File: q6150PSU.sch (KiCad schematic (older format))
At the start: 25 parts, among them P1 Vin, P2 Vout, P3 CONN_01X03, Q1 Q_NMOS_GSD, T1 TRANSFO, U1 LM3478

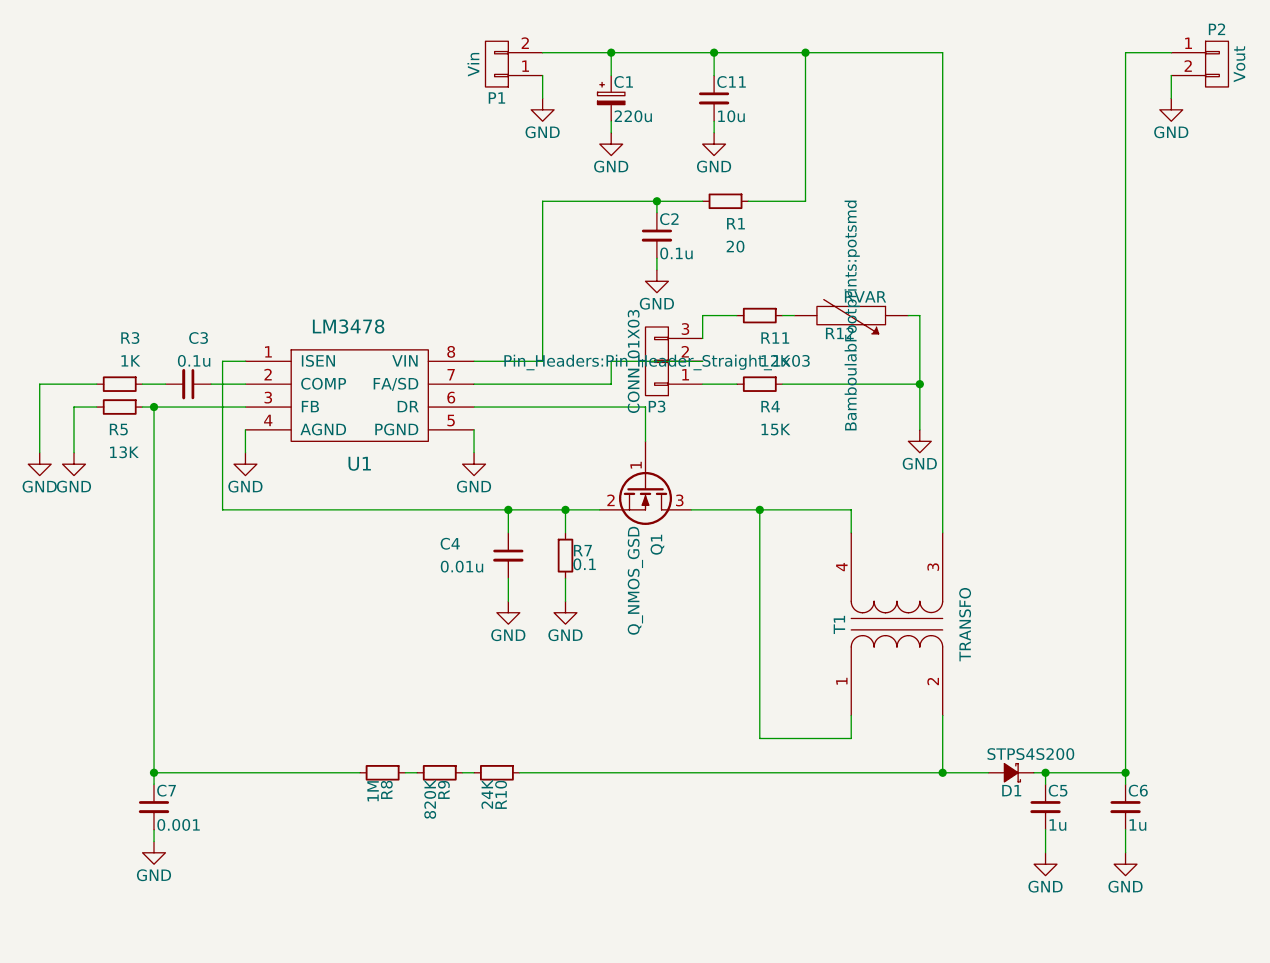
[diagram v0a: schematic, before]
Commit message: Fixed and it works!
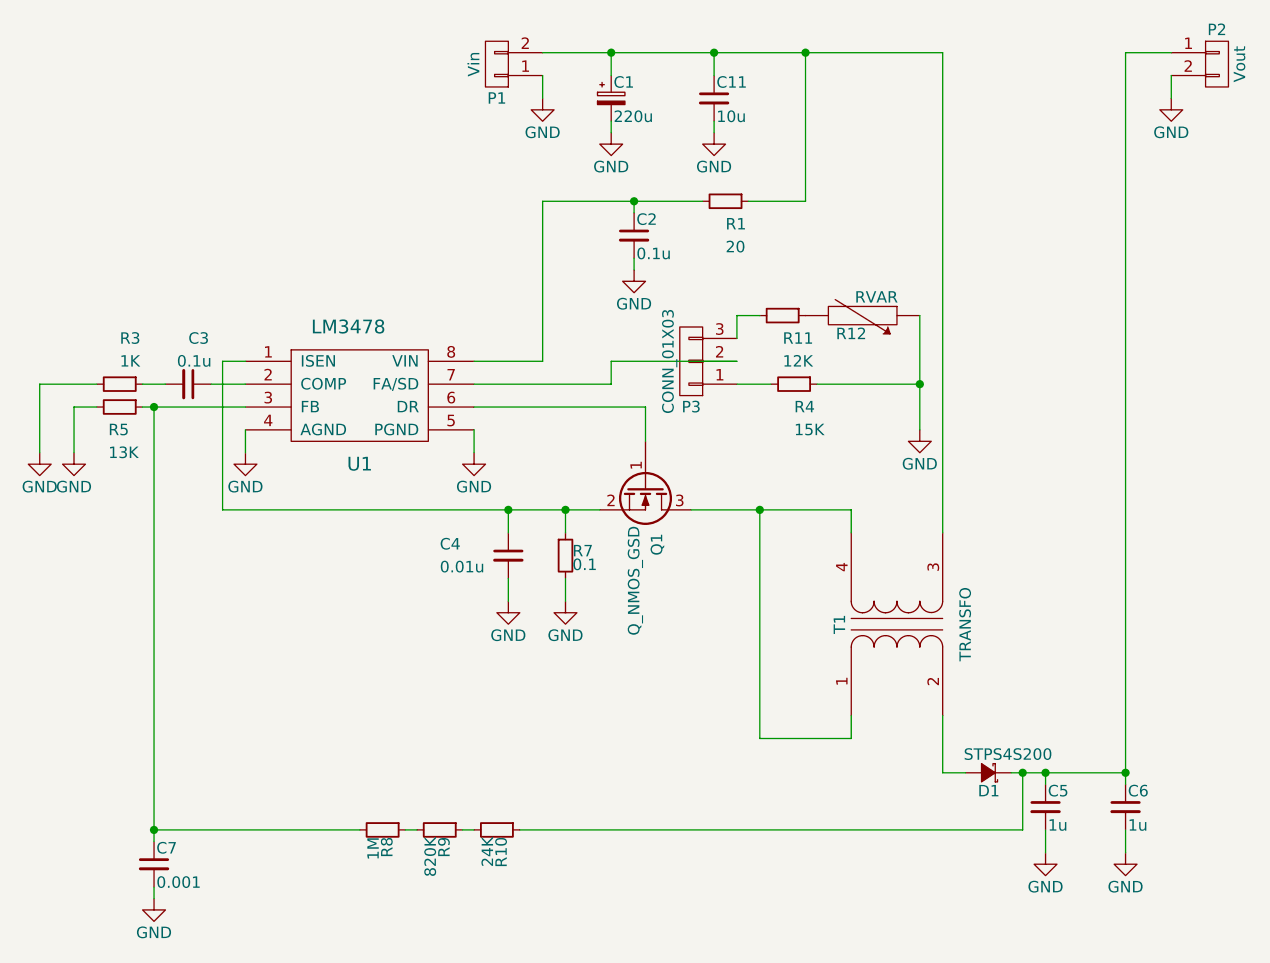
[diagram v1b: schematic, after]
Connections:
- net at C5.1, C6.1, D1.1 (K)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: now also R10.1
- net at D1.2 (A), T1.2 (AB): no longer R10.1
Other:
- moved on the sheet: C2, C7, D1, P3, R10, R11, R12, R4, R8, R9
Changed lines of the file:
@@
 L C_Small C2
 U 1 1 57F6A28E
-P 4900 2700
-F 0 "C2" H 4910 2770 50  0000 L CNN
-F 1 "0.1u" H 4910 2620 50  0000 L CNN
-F 2 "Capacitors_SMD:C_0805_HandSoldering" H 4900 2700 50  0001 C CNN
-F 3 "" H 4900 2700 50  0000 C CNN
-	1    4900 2700
+P 4800 2700
+F 0 "C2" H 4810 2770 50  0000 L CNN
+F 1 "0.1u" H 4810 2620 50  0000 L CNN
+F 2 "Capacitors_SMD:C_0805_HandSoldering" H 4800 2700 50  0001 C CNN
+F 3 "" H 4800 2700 50  0000 C CNN
+	1    4800 2700
 	1    0    0    -1
 $EndComp
@@
 L GND #PWR04
 U 1 1 57F6A2BF
-P 4900 2850
-F 0 "#PWR04" H 4900 2600 50  0001 C CNN
-F 1 "GND" H 4900 2700 50  0000 C CNN
-F 2 "" H 4900 2850 50  0000 C CNN
-F 3 "" H 4900 2850 50  0000 C CNN
-	1    4900 2850
+P 4800 2850
+F 0 "#PWR04" H 4800 2600 50  0001 C CNN
+F 1 "GND" H 4800 2700 50  0000 C CNN
+F 2 "" H 4800 2850 50  0000 C CNN
+F 3 "" H 4800 2850 50  0000 C CNN
+	1    4800 2850
 	1    0    0    -1
 $EndComp
@@
 L R_Small R4
 U 1 1 57F6BD03
-P 5350 3350
-F 0 "R4" V 5450 3350 50  0000 L CNN
-F 1 "15K" V 5550 3350 50  0000 L CNN
-F 2 "Resistors_SMD:R_0805_HandSoldering" H 5350 3350 50  0001 C CNN
-F 3 "" H 5350 3350 50  0000 C CNN
-	1    5350 3350
+P 5500 3350
+F 0 "R4" V 5600 3350 50  0000 L CNN
+F 1 "15K" V 5700 3350 50  0000 L CNN
+F 2 "Resistors_SMD:R_0805_HandSoldering" H 5500 3350 50  0001 C CNN
+F 3 "" H 5500 3350 50  0000 C CNN
+	1    5500 3350
 	0    1    1    0
 $EndComp
@@
 L D_Schottky_Small D1
 U 1 1 57F6D48D
-P 6450 5050
-F 0 "D1" H 6400 5130 50  0000 L CNN
-F 1 "STPS4S200" H 6170 4970 50  0000 L CNN
-F 2 "Diodes_SMD:SMB_Handsoldering" V 6450 5050 50  0001 C CNN
-F 3 "" V 6450 5050 50  0000 C CNN
-	1    6450 5050
+P 6350 5050
+F 0 "D1" H 6300 5130 50  0000 L CNN
+F 1 "STPS4S200" H 6070 4970 50  0000 L CNN
+F 2 "Diodes_SMD:SMB_Handsoldering" V 6350 5050 50  0001 C CNN
+F 3 "" V 6350 5050 50  0000 C CNN
+	1    6350 5050
 	-1   0    0    1
 $EndComp
@@
 L GND #PWR014
 U 1 1 57F6E467
-P 2700 5350
-F 0 "#PWR014" H 2700 5100 50  0001 C CNN
-F 1 "GND" H 2700 5200 50  0000 C CNN
-F 2 "" H 2700 5350 50  0000 C CNN
-F 3 "" H 2700 5350 50  0000 C CNN
-	1    2700 5350
+P 2700 5600
+F 0 "#PWR014" H 2700 5350 50  0001 C CNN
+F 1 "GND" H 2700 5450 50  0000 C CNN
+F 2 "" H 2700 5600 50  0000 C CNN
+F 3 "" H 2700 5600 50  0000 C CNN
+	1    2700 5600
 	1    0    0    -1
 $EndComp
@@
 L C_Small C7
 U 1 1 57F6E4A1
-P 2700 5200
-F 0 "C7" H 2710 5270 50  0000 L CNN
-F 1 "0.001" H 2710 5120 50  0000 L CNN
-F 2 "Capacitors_SMD:C_0805_HandSoldering" H 2700 5200 50  0001 C CNN
-F 3 "" H 2700 5200 50  0000 C CNN
-	1    2700 5200
+P 2700 5450
+F 0 "C7" H 2710 5520 50  0000 L CNN
+F 1 "0.001" H 2710 5370 50  0000 L CNN
+F 2 "Capacitors_SMD:C_0805_HandSoldering" H 2700 5450 50  0001 C CNN
+F 3 "" H 2700 5450 50  0000 C CNN
+	1    2700 5450
 	1    0    0    -1
 $EndComp
@@
 L R_Small R8
 U 1 1 57F6E5C7
-P 3700 5050
-F 0 "R8" H 3730 5070 50  0000 L CNN
-F 1 "1M" H 3730 5010 50  0000 L CNN
-F 2 "Resistors_SMD:R_0805_HandSoldering" H 3700 5050 50  0001 C CNN
-F 3 "" H 3700 5050 50  0000 C CNN
-	1    3700 5050
+P 3700 5300
+F 0 "R8" H 3730 5320 50  0000 L CNN
+F 1 "1M" H 3730 5260 50  0000 L CNN
+F 2 "Resistors_SMD:R_0805_HandSoldering" H 3700 5300 50  0001 C CNN
+F 3 "" H 3700 5300 50  0000 C CNN
+	1    3700 5300
 	0    1    1    0
 $EndComp
@@
 L R_Small R9
 U 1 1 57F6E6A8
-P 3950 5050
-F 0 "R9" H 3980 5070 50  0000 L CNN
-F 1 "820K" H 3980 5010 50  0000 L CNN
-F 2 "Resistors_SMD:R_0805_HandSoldering" H 3950 5050 50  0001 C CNN
-F 3 "" H 3950 5050 50  0000 C CNN
-	1    3950 5050
+P 3950 5300
+F 0 "R9" H 3980 5320 50  0000 L CNN
+F 1 "820K" H 3980 5260 50  0000 L CNN
+F 2 "Resistors_SMD:R_0805_HandSoldering" H 3950 5300 50  0001 C CNN
+F 3 "" H 3950 5300 50  0000 C CNN
+	1    3950 5300
 	0    1    1    0
 $EndComp
@@
 L R_Small R10
 U 1 1 57F6E6EB
-P 4200 5050
-F 0 "R10" H 4230 5070 50  0000 L CNN
-F 1 "24K" H 4230 5010 50  0000 L CNN
-F 2 "Resistors_SMD:R_0805_HandSoldering" H 4200 5050 50  0001 C CNN
-F 3 "" H 4200 5050 50  0000 C CNN
-	1    4200 5050
+P 4200 5300
+F 0 "R10" H 4230 5320 50  0000 L CNN
+F 1 "24K" H 4230 5260 50  0000 L CNN
+F 2 "Resistors_SMD:R_0805_HandSoldering" H 4200 5300 50  0001 C CNN
+F 3 "" H 4200 5300 50  0000 C CNN
+	1    4200 5300
 	0    1    1    0
 $EndComp
@@
 	5150 2200 5150 2250
 Wire Wire Line
-	4900 2800 4900 2850
+	4800 2800 4800 2850
 Wire Wire Line
 	5300 2550 5550 2550
@@
 	4400 2550 5100 2550
 Wire Wire Line
-	4900 2550 4900 2600
+	4800 2550 4800 2600
 Wire Wire Line
 	4400 2550 4400 3250
 Wire Wire Line
 	4400 3250 4100 3250
-Connection ~ 4900 2550
+Connection ~ 4800 2550
 Connection ~ 5550 1900
 Wire Wire Line
@@
 	6950 1900 6950 5100
 Wire Wire Line
-	6550 5050 6950 5050
-Wire Wire Line
-	4300 5050 6350 5050
+	6450 5050 6950 5050
+Wire Wire Line
+	6150 5050 6250 5050
 Wire Wire Line
 	7150 2000 7150 2100
@@
 Connection ~ 6600 5050
 Wire Wire Line
-	2700 3450 2700 5100
+	2700 3450 2700 5350
 Connection ~ 2700 3450
 Wire Wire Line
-	2700 5300 2700 5350
-Connection ~ 6150 5050
-Wire Wire Line
-	4100 5050 4050 5050
-Wire Wire Line
-	3850 5050 3800 5050
-Wire Wire Line
-	5100 3350 5250 3350
+	2700 5550 2700 5600
+Wire Wire Line
+	4100 5300 4050 5300
+Wire Wire Line
+	3850 5300 3800 5300
+Wire Wire Line
+	5250 3350 5400 3350
 $Comp
 L GND #PWR015
@@
 $EndComp
 Wire Wire Line
-	5450 3350 6050 3350
-Wire Wire Line
-	3600 5050 2700 5050
-Connection ~ 2700 5050
+	5600 3350 6050 3350
+Wire Wire Line
+	3600 5300 2700 5300
+Connection ~ 2700 5300
 Wire Wire Line
 	5750 3900 5750 4000
@@
 L R_Small R11
 U 1 1 58020BA0
-P 5350 3050
-F 0 "R11" V 5450 3050 50  0000 L CNN
-F 1 "12K" V 5550 3050 50  0000 L CNN
-F 2 "Resistors_SMD:R_0805_HandSoldering" H 5350 3050 50  0001 C CNN
-F 3 "" H 5350 3050 50  0000 C CNN
-	1    5350 3050
+P 5450 3050
+F 0 "R11" V 5550 3050 50  0000 L CNN
+F 1 "12K" V 5650 3050 50  0000 L CNN
+F 2 "Resistors_SMD:R_0805_HandSoldering" H 5450 3050 50  0001 C CNN
+F 3 "" H 5450 3050 50  0000 C CNN
+	1    5450 3050
 	0    1    1    0
 $EndComp
@@
 L RVAR R12
 U 1 1 58021FB9
-P 5750 3050
-F 0 "R12" V 5830 3000 50  0000 C CNN
-F 1 "RVAR" V 5670 3110 50  0000 C CNN
-F 2 "BamboulabFootprints:potsmd" H 5750 3050 50  0000 C CNN
-F 3 "" H 5750 3050 50  0000 C CNN
-	1    5750 3050
-	0    1    1    0
-$EndComp
-Wire Wire Line
-	5100 3050 5250 3050
-Wire Wire Line
-	5450 3050 5500 3050
-Wire Wire Line
-	6000 3050 6050 3050
+P 5800 3050
+F 0 "R12" V 5880 3000 50  0000 C CNN
+F 1 "RVAR" V 5720 3110 50  0000 C CNN
+F 2 "BamboulabFootprints:potsmd" H 5800 3050 50  0001 C CNN
+F 3 "" H 5800 3050 50  0000 C CNN
+	1    5800 3050
+	0    1    1    0
+$EndComp
+Wire Wire Line
+	5250 3050 5350 3050
+Wire Wire Line
+	5550 3050 5550 3050
 Connection ~ 6050 3350
 $Comp
 L CONN_01X03 P3
 U 1 1 58022C9D
-P 4900 3250
-F 0 "P3" H 4900 3450 50  0000 C CNN
-F 1 "CONN_01X03" V 5000 3250 50  0000 C CNN
-F 2 "Pin_Headers:Pin_Header_Straight_1x03" H 4900 3250 50  0000 C CNN
-F 3 "" H 4900 3250 50  0000 C CNN
-	1    4900 3250
+P 5050 3250
+F 0 "P3" H 5050 3450 50  0000 C CNN
+F 1 "CONN_01X03" V 5150 3250 50  0000 C CNN
+F 2 "Pin_Headers:Pin_Header_Straight_1x03" H 5050 3250 50  0001 C CNN
+F 3 "" H 5050 3250 50  0000 C CNN
+	1    5050 3250
 	-1   0    0    1
 $EndComp
 Wire Wire Line
-	5100 3150 5100 3050
+	5250 3150 5250 3050
 Wire Wire Line
 	4100 3350 4700 3350
@@
 	4700 3350 4700 3250
 Wire Wire Line
-	4700 3250 5100 3250
+	4700 3250 5250 3250
+Wire Wire Line
+	4300 5300 6500 5300
+Wire Wire Line
+	6500 5300 6500 5050
+Connection ~ 6500 5050
 $EndSCHEMATC
